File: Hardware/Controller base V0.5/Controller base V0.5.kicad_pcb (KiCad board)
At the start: 2 copper layers, 63.2 x 68.5 mm, 35 parts, among them J1 USB_C_Receptacle_USB2.0_16P, J2 Conn_01x05_Pin, J3 right face mod, J4 left face mod, J5 left sholder, J6 right sholder, SW1 SW_Push, SW2 SW_Push, SW3 SW_Push, SW4 SW_Push, U1 AZ1117CH-3.3TRG1, U2 ESP32-S3-WROOM-1U-N4

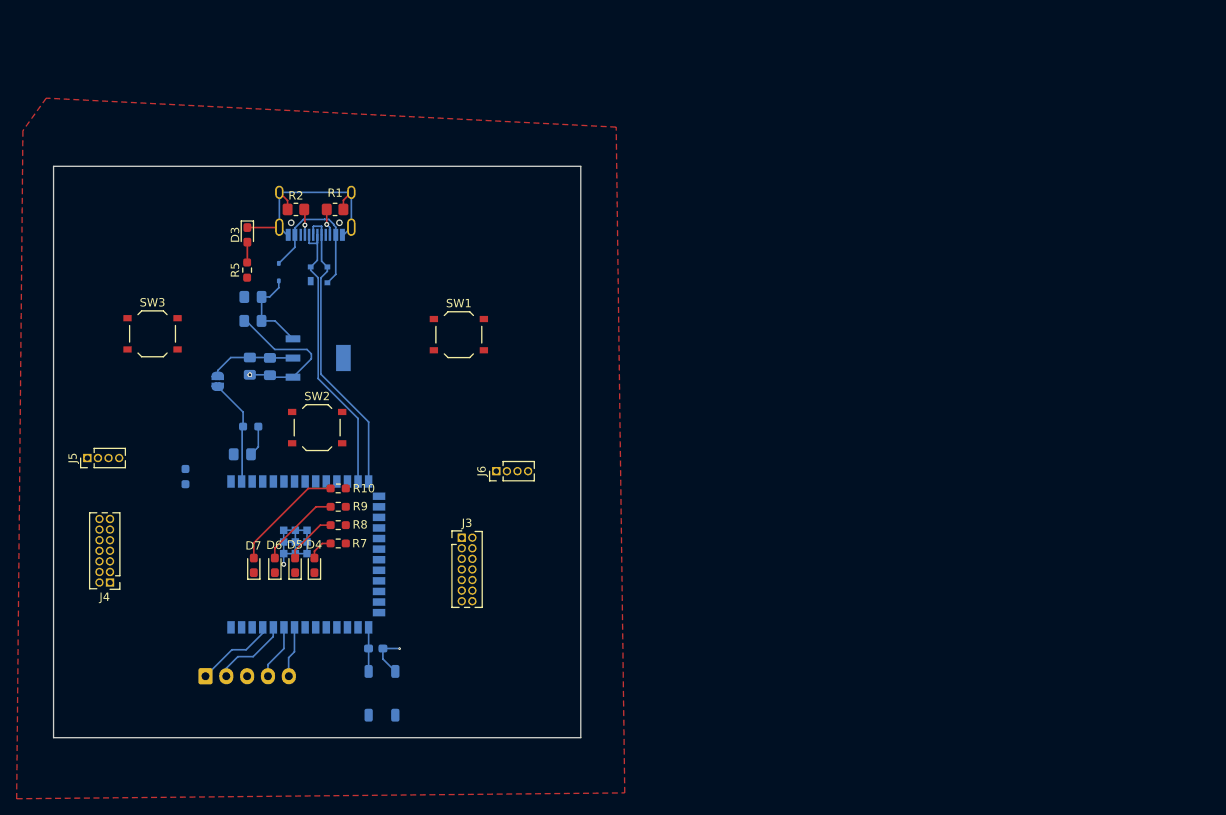
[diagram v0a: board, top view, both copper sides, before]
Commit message: update
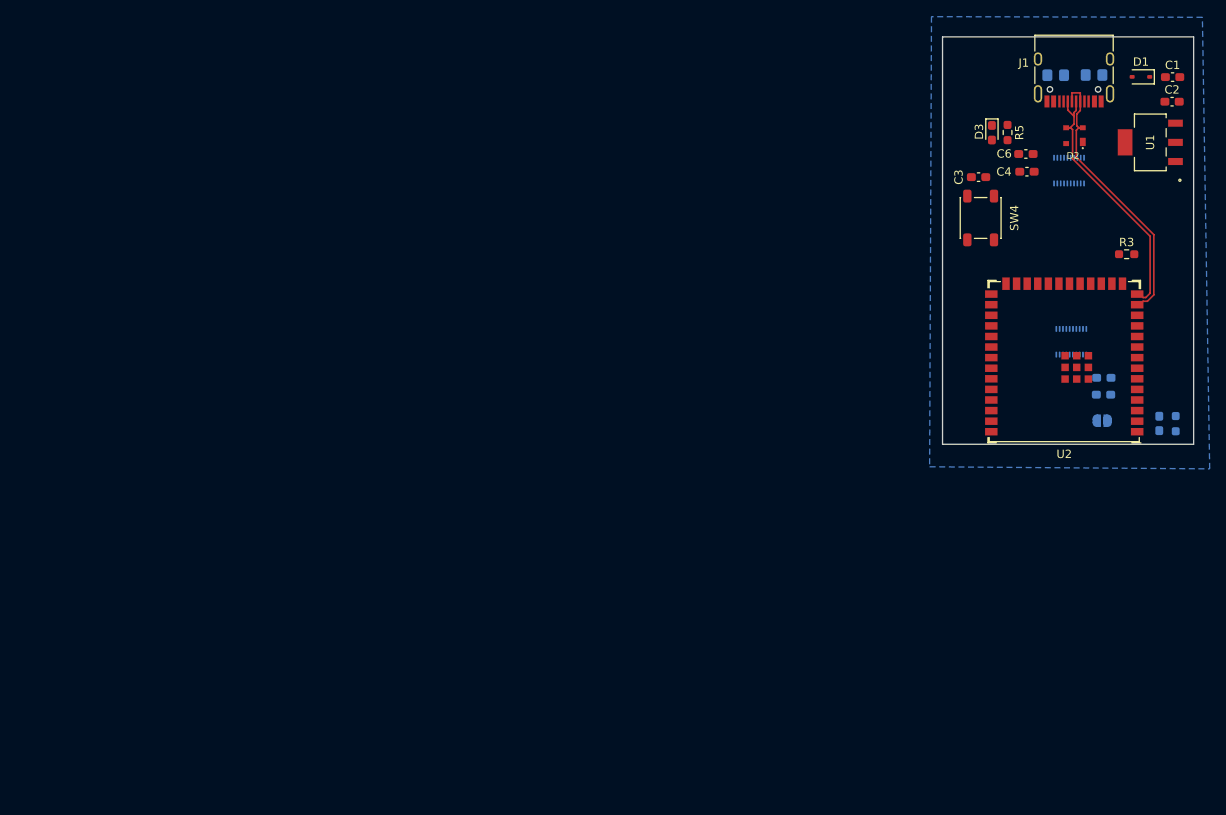
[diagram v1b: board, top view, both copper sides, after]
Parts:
- removed D4, D5, D6, D7: LED, LED_SMD:LED_0603_1608Metric_Pad1.05x0.95mm_HandSolder
- removed J2: Conn_01x05_Pin, Connector_JST:JST_EH_S5B-EH_1x05_P2.50mm_Horizontal
- removed J3: right face mod, Connector_PinHeader_1.27mm:PinHeader_2x07_P1.27mm_Vertical
- removed J4: left face mod, Connector_PinHeader_1.27mm:PinHeader_2x07_P1.27mm_Vertical
- removed J5: left sholder, Connector_PinHeader_1.27mm:PinHeader_1x04_P1.27mm_Vertical
- removed J6: right sholder, Connector_PinHeader_1.27mm:PinHeader_1x04_P1.27mm_Vertical
- removed R10, R7, R8, R9: 1K, Resistor_SMD:R_0603_1608Metric_Pad0.98x0.95mm_HandSolder
- removed SW1, SW2, SW3: SW_Push, Button_Switch_SMD:SW_Push_1P1T_XKB_TS-1187A
- added C5: 10uF, Capacitor_SMD:C_0603_1608Metric_Pad1.08x0.95mm_HandSolder, B.Cu at (241.8, 98.5)
- added C7: 0.1uF, Capacitor_SMD:C_0603_1608Metric_Pad1.08x0.95mm_HandSolder, B.Cu at (241.8, 100.5)
- added J7: Conn_02x10_Counter_Clockwise, Connector_Hirose_DF40:Hirose_DF40C-20DS-0.4V_2x10_P0.4mm, B.Cu at (237.7, 73.7)
- added J8: Conn_02x10_Counter_Clockwise, Connector_Hirose_DF40:Hirose_DF40C-20DS-0.4V_2x10_P0.4mm, B.Cu at (237.9, 94.2)
- C1, C2, C4, C6: footprint Capacitor_SMD:C_0805_2012Metric_Pad1.18x1.45mm_HandSolder -> Capacitor_SMD:C_0603_1608Metric_Pad1.08x0.95mm_HandSolder; moved to F.Cu
- C3, D1, D2, J1, R3, SW4, U1, U2: moved to F.Cu
- C8: footprint Capacitor_SMD:C_0805_2012Metric_Pad1.18x1.45mm_HandSolder -> Capacitor_SMD:C_0603_1608Metric_Pad1.08x0.95mm_HandSolder
- R1, R2: moved to B.Cu
- moved R3 116.0 mm to (244.6, 83.7), turned to 0 degrees
- moved C1 113.4 mm to (250.1, 62.5), turned to 0 degrees
- moved C2 113.4 mm to (250.0, 65.4), turned to 0 degrees
- moved R4 111.0 mm to (250.4, 104.0), turned to -90 degrees
- moved C8 110.1 mm to (248.5, 104.0), turned to -90 degrees
- moved R6 106.2 mm to (241.6, 103.7), turned to 0 degrees
- moved D1 106.0 mm to (246.3, 62.4), turned to 180 degrees
- moved U1 103.1 mm to (247.4, 70.3)
- moved R2 97.1 mm to (240.7, 62.2), turned to 180 degrees
- moved C4 96.1 mm to (232.6, 73.8), turned to 180 degrees
- moved U2 94.5 mm to (237.1, 96.7), turned to 180 degrees
- moved C6 94.2 mm to (232.5, 71.7), turned to 180 degrees
- moved R5 92.7 mm to (230.3, 69.1), turned to -90 degrees
- moved J1 92.4 mm to (238.2, 61.3), turned to 180 degrees
- moved D2 92.2 mm to (238.3, 69.5)
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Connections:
- U2 pad 8: GPIO1 -> GPIO15
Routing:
- net GND: track 70.8 -> 0.00 mm, vias 3 -> 0
- net VBUS: track 17.9 -> 0.00 mm
- net Net-(D7-A): track 13.7 -> 0.00 mm
- net ESP_3.3V: track 12.7 -> 0.00 mm
- net VCC_5V: track 10.9 -> 0.00 mm
- net VCC_3V3: track 10.3 -> 0.00 mm
- net Net-(D6-A): track 9.94 -> 0.00 mm
- net TXD0: track 9.70 -> 0.00 mm
- net RXD0: track 9.28 -> 0.00 mm
- net GPIO42: track 6.65 -> 0.00 mm
- net Net-(D5-A): track 6.44 -> 0.00 mm
- net GPIO41: track 6.16 -> 0.00 mm
- net GPIO0: track 5.28 -> 0.00 mm
- net D+: track 35.6 -> 31.7 mm
- net /CHIP_PU: track 3.69 -> 0.00 mm
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- added copper zone on B.Cu, net GND
- removed copper zone on F.Cu, net GND
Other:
- board size 63.2 x 68.5 mm -> 30.1 x 48.9 mm
